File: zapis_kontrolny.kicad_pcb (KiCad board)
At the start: 2 copper layers, 49.5 x 49.5 mm, 67 parts, among them P1 CONN_01X06, P10 M1, P11 M2, P12 CONN_01X02, P2 CONN_01X06, P3 CONN_01X06, P4 CONN_01X06, P5 UART, P6 CONN_01X05, P7 CONN_01X02, Q1 IRF9540N, U1 74AHC1G14, U10 HL293D, U2 TLP291, U3 TLP291, U4 LM7812CT, U5 74AHC1G14, U6 STM32F103C6Tx, U7 LM7805CT, U8 LM1117-3.3, U9 HL293D

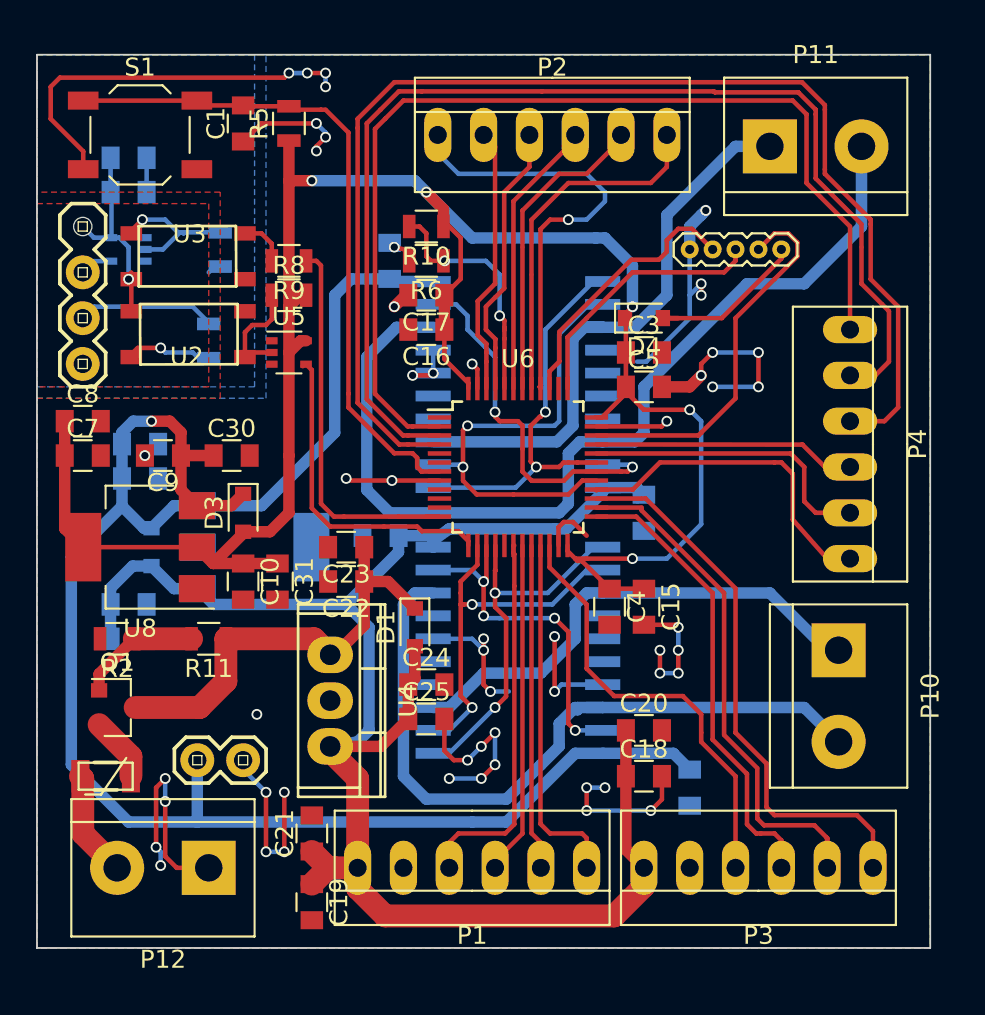
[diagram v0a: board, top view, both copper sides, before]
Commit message: final
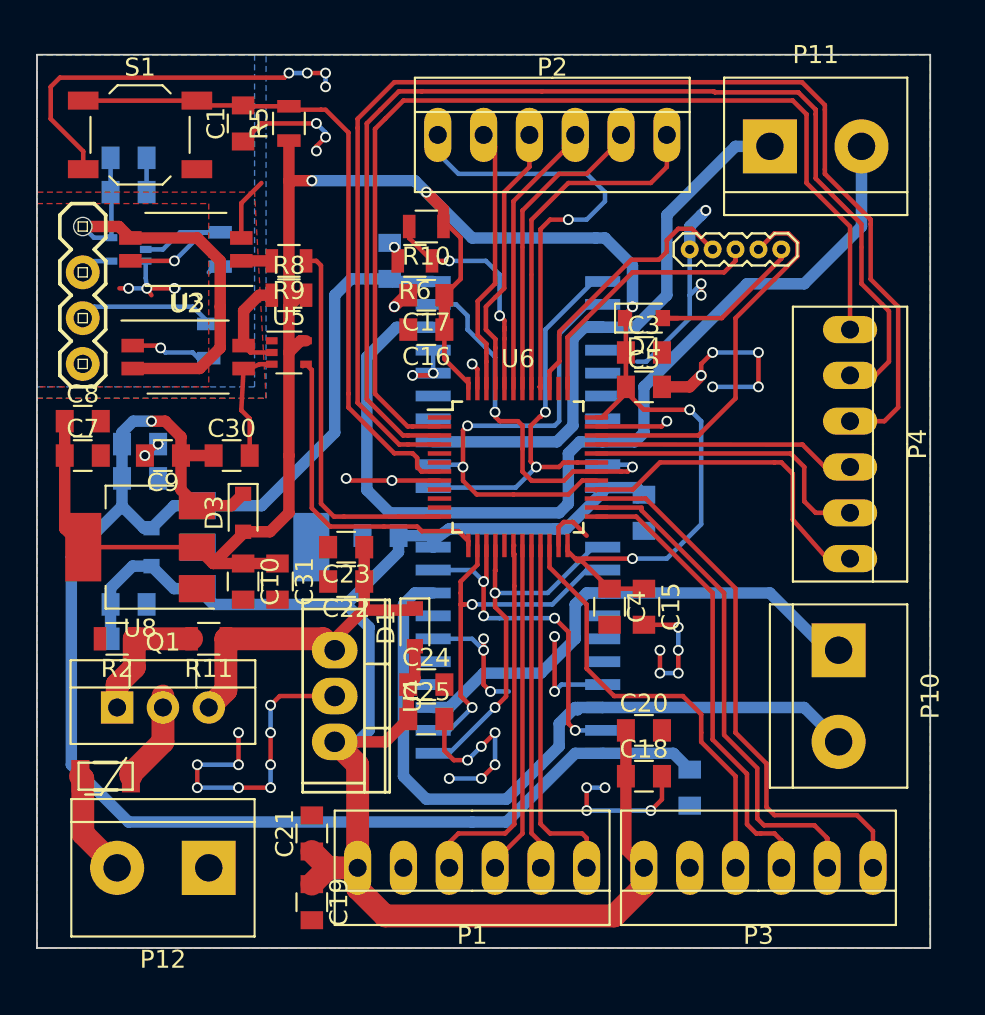
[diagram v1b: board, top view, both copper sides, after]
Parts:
- removed P7: CONN_01X02, SparkFun:SparkFun-1X02
- Q1: footprint TO_SOT_Packages_SMD:SOT-23 -> TO_SOT_Packages_THT:TO-220_Vertical
- U2, U3: value TLP291 -> LTV-358T; footprint MyLib:Gul_wings_4 -> Buttons_Switches_SMD:SW_DIP_x2_W6.15mm_Slide_Omron_A6H
- moved U3 1.27 mm to (196.3, 67.6), turned to 0 degrees
- moved R6 0.64 mm to (208.9, 62.2)
- moved U2 0.40 mm to (196.2, 61.6), turned to 180 degrees
- moved U4 0.36 mm to (204.5, 86.4)
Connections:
- U2 pad 1: Net-(R7-Pad1) -> Net-(R9-Pad2)
- U2 pad 2: VSS -> GND
- U2 pad 3: GND -> VSS
- U2 pad 4: Net-(R9-Pad2) -> Net-(R7-Pad1)
- U3 pad 1: Net-(R8-Pad1) -> Net-(R1-Pad1)
- U3 pad 2: GND -> VSS
- U3 pad 3: VSS -> GND
- U3 pad 4: Net-(R1-Pad1) -> Net-(R8-Pad1)
- U6 pad 10: (no net) -> /Enc0
- U6 pad 11: (no net) -> /Enc1
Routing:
- net VSS: track 11.9 -> 24.9 mm, vias 1 -> 0
- net GND: track 131.7 -> 137.5 mm, vias 52 -> 54
- net VEE: track 3.31 -> 8.58 mm, vias 0 -> 3
- net Net-(C22-Pad1): track 24.6 -> 19.8 mm
- net +5C: track 102.0 -> 98.1 mm, vias 2 -> 1
- net Net-(R7-Pad1): track 8.20 -> 10.2 mm
- net Net-(F1-Pad1): track 3.59 -> 5.18 mm
- net Net-(R9-Pad2): track 3.15 -> 1.69 mm
- net Net-(Q1-Pad1): track 6.85 -> 7.38 mm
- net (no net): vias 1 -> 0
